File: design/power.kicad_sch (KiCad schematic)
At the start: 56 parts, among them J1 POWER, U1 LM3880MF-1AA, U2 NCP59744MN1, U3 NCP59744MN1, U4 NCP59744MN1, U5 NCP59744MN1

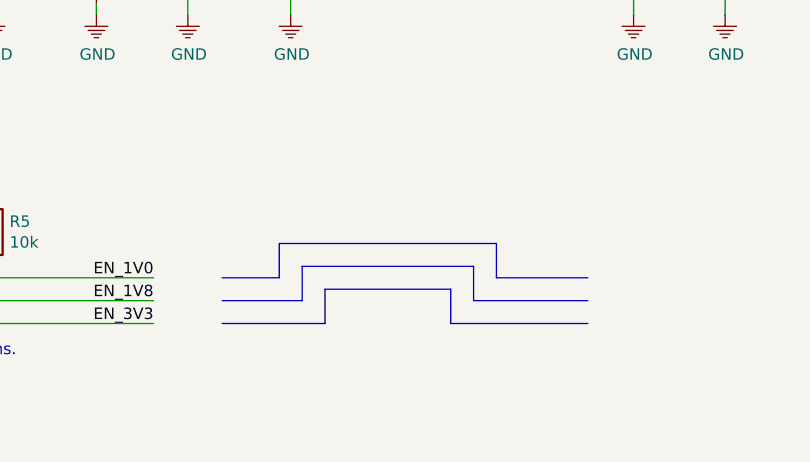
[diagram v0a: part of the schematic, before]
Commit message: Updated LNA
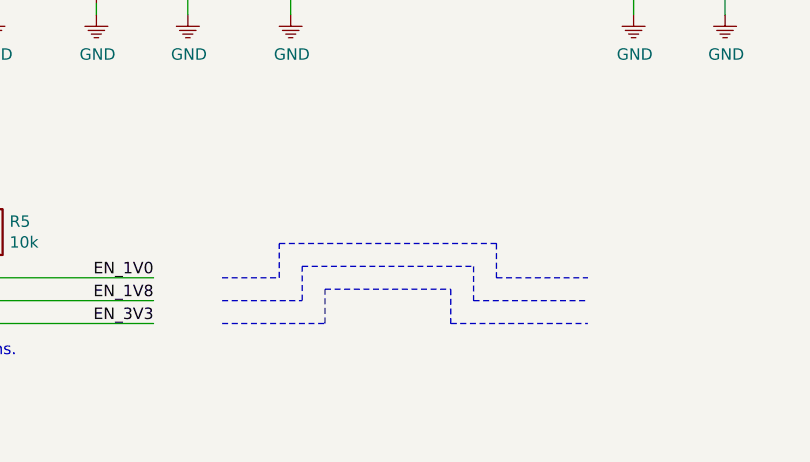
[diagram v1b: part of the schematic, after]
